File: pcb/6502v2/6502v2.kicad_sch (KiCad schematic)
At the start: 4 parts, among them J1 Power, U1 74HC00, U2 74HC238, X1 DGOF5S3

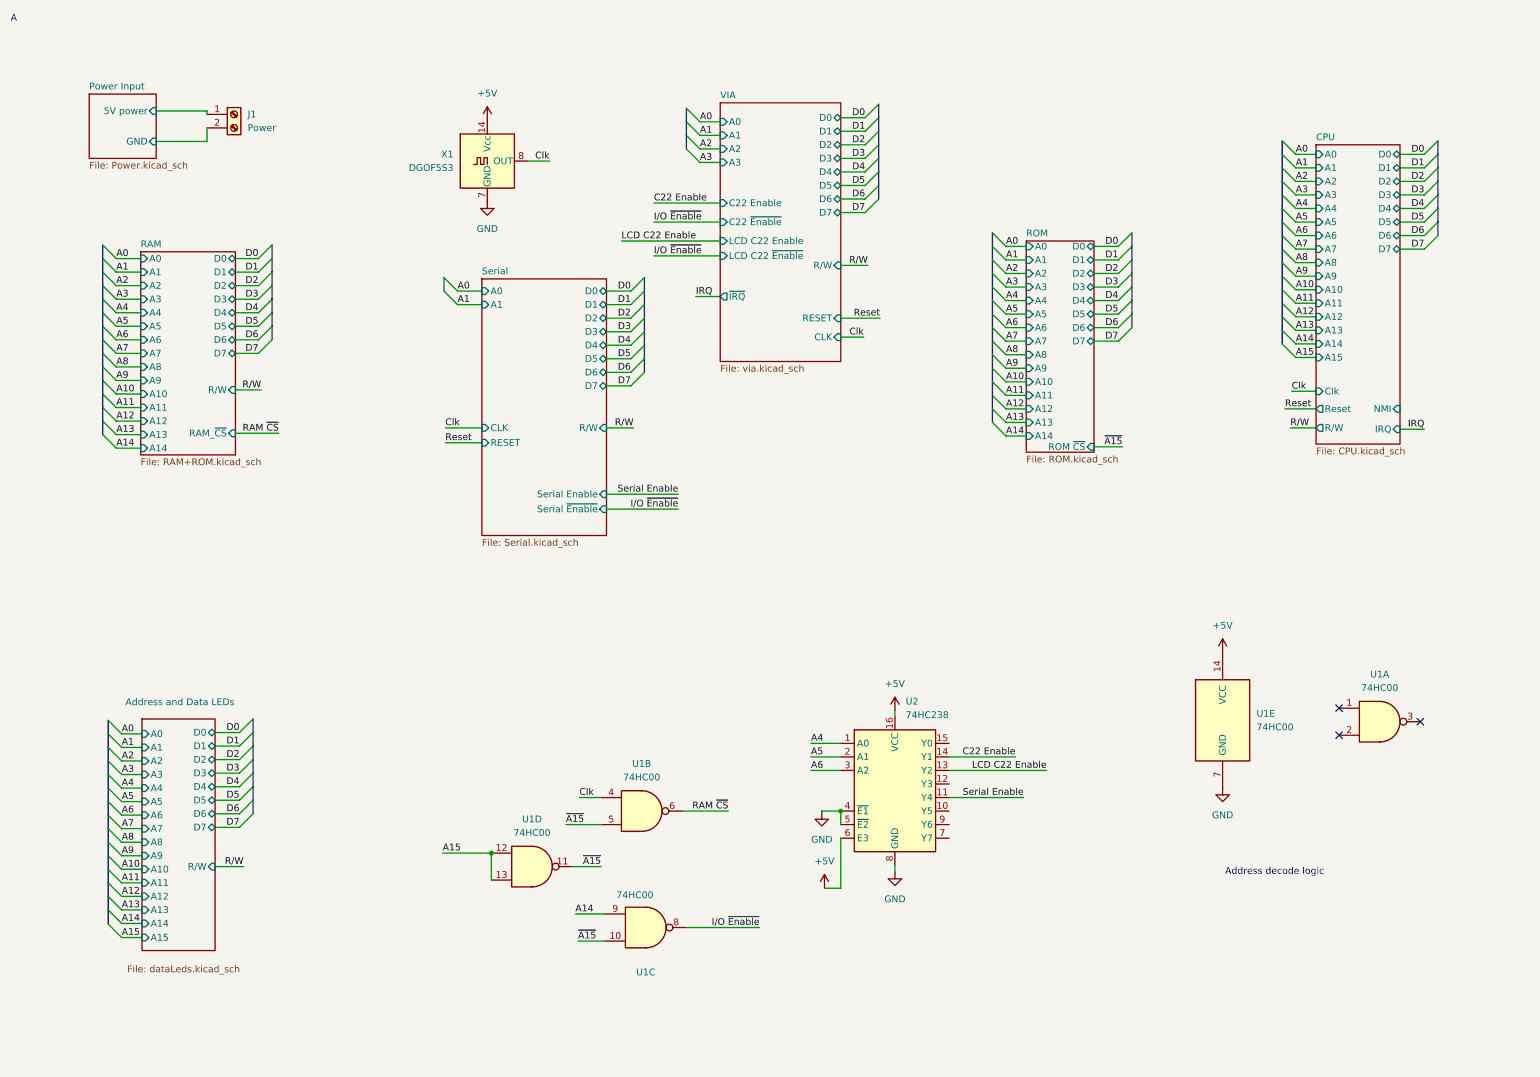
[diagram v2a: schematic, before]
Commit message: Tidying up schematic
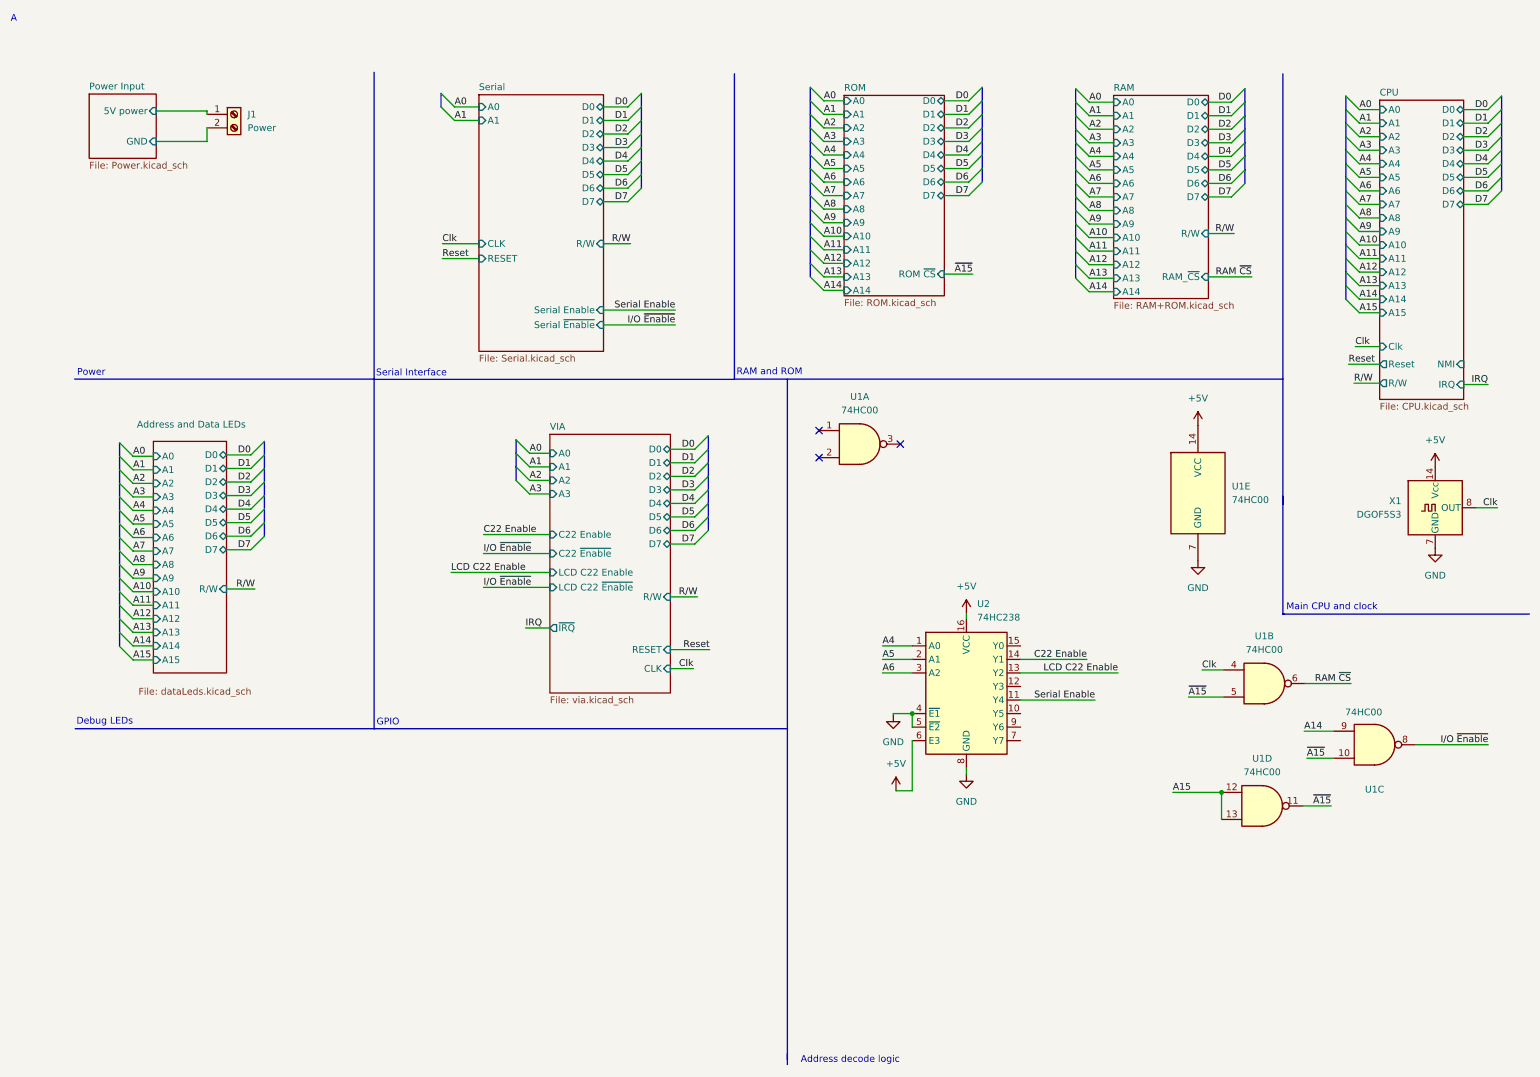
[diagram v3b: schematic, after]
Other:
- note added: "Debug LEDs"
- note added: "GPIO"
- note added: "Main CPU and clock"
- note added: "Power"
- note added: "RAM and ROM"
- note added: "Serial Interface"
- moved on the sheet: U1A, U1B, U1C, U1D, U1E, U2, X1
